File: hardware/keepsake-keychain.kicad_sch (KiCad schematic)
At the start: 3 parts

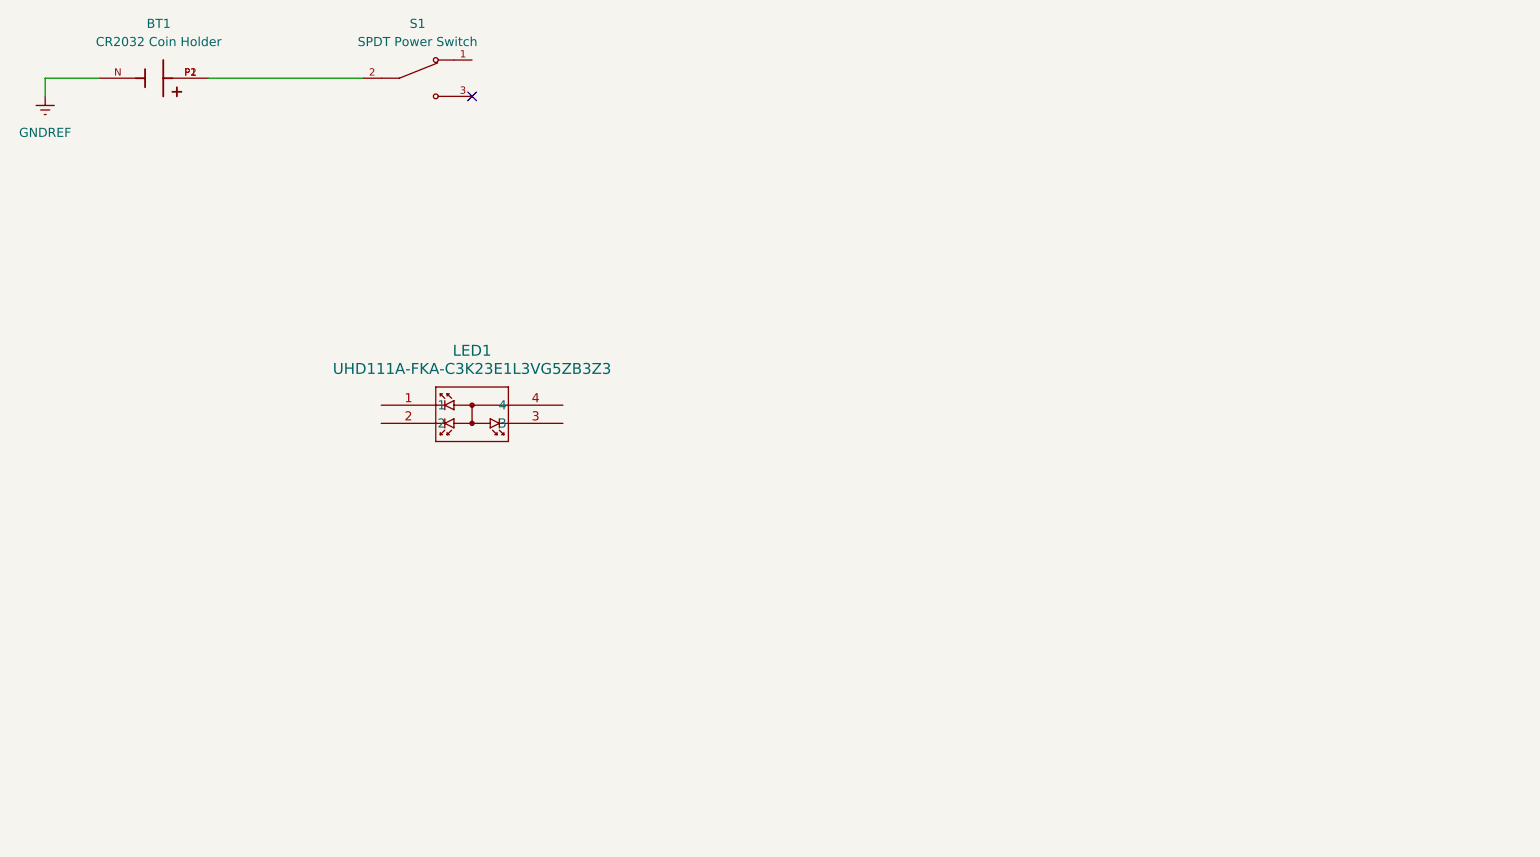
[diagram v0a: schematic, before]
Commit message: Add ATtiny1614 IC
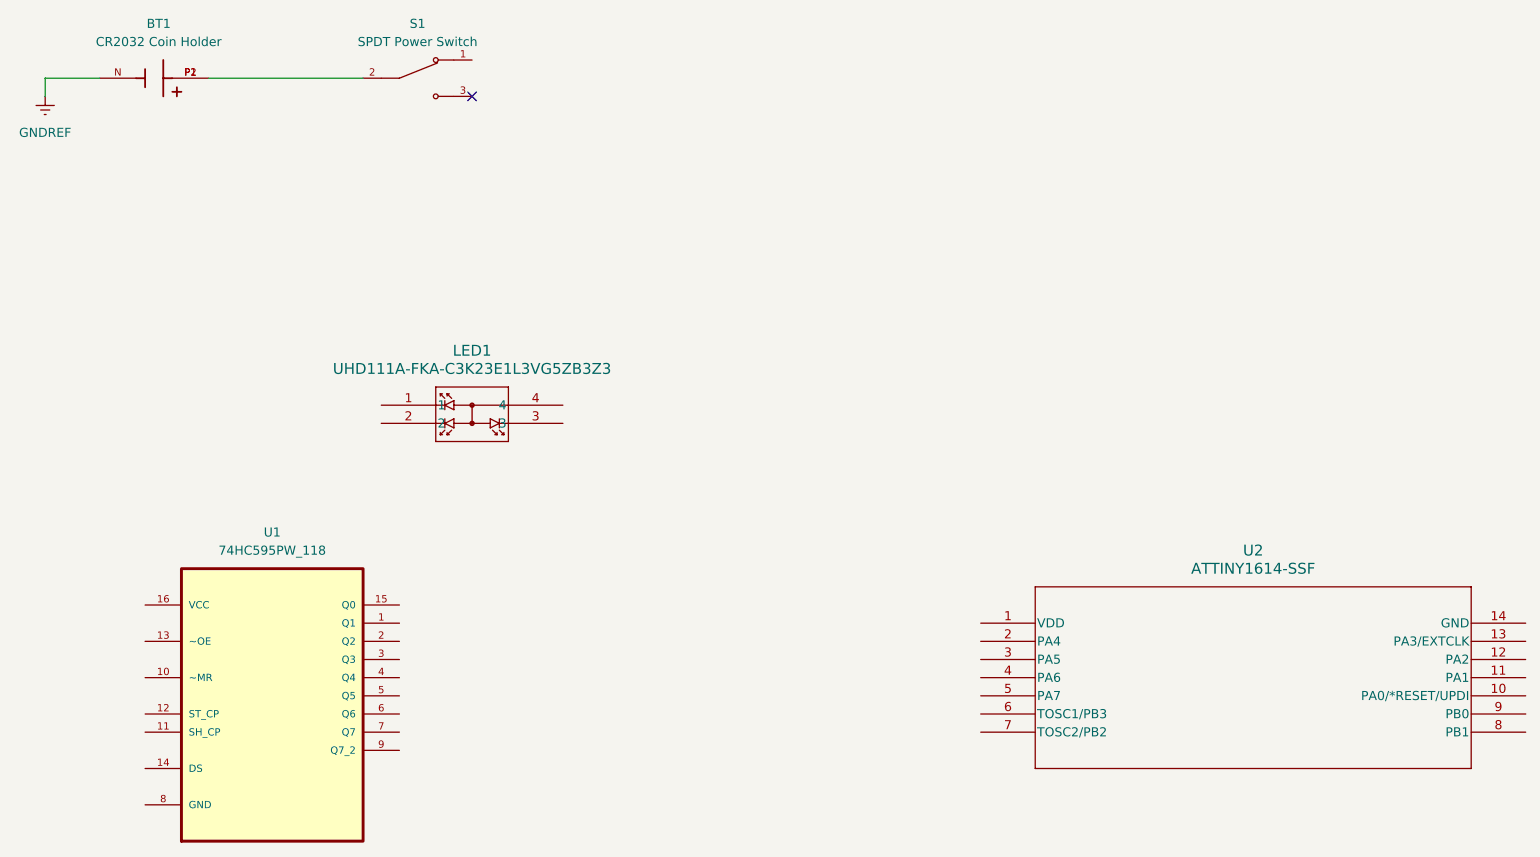
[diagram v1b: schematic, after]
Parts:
- added U1: 74HC595PW_118, 74HC595PW_118:SOP65P640X110-16N, symbol 0_74HC595_Shift_Register:74HC595PW_118
- added U2: ATTINY1614-SSF, SOIC14_SL_MCH, symbol 0_ATtiny1614:ATTINY1614-SSF
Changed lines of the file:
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@@
+	)
+	(symbol
+		(lib_id "0_ATtiny1614:ATTINY1614-SSF")
+		(at 176.53 127 0)
+		(unit 1)
+		(exclude_from_sim no)
+		(in_bom yes)
+		(on_board yes)
+		(dnp no)
+		(fields_autoplaced yes)
+		(property "Reference" "U2"
+			(at 214.63 116.84 0)
+			(effects
+				(font
+					(size 1.524 1.524)
+				)
+			)
+		)
+		(property "Value" "ATTINY1614-SSF"
+			(at 214.63 119.38 0)
+			(effects
+				(font
+					(size 1.524 1.524)
+				)
+			)
+		)
+		(property "Footprint" "SOIC14_SL_MCH"
+			(at 176.53 127 0)
+			(effects
+				(font
+					(size 1.27 1.27)
+					(italic yes)
+				)
+				(hide yes)
+			)
+		)
+		(property "Datasheet" "ATTINY1614-SSF"
+			(at 176.53 127 0)
+			(effects
+				(font
+					(size 1.27 1.27)
+					(italic yes)
+				)
+				(hide yes)
+			)
+		)
+		(property "Description" ""
+			(at 176.53 127 0)
+			(effects
+				(font
+					(size 1.27 1.27)
+				)
+				(hide yes)
+			)
+		)
+		(pin "3"
+		)
+		(pin "1"
+		)
+		(pin "2"
+		)
+		(pin "6"
+		)
+		(pin "8"
+		)
+		(pin "4"
+		)
+		(pin "14"
+		)
+		(pin "12"
+		)
+		(pin "9"
+		)
+		(pin "13"
+		)
+		(pin "10"
+		)
+		(pin "7"
+		)
+		(pin "5"
+		)
+		(pin "11"
+		)
+		(instances
+			(project ""
+				(path "/32670795-e352-430d-9b7f-c7f10ebe6399"
+					(reference "U2")
+					(unit 1)
+				)
+			)
+		)
 	)
 	(symbol
@@
 					(unit 1)
 				)
+			)
+		)
+	)
+	(symbol
+		(lib_id "0_74HC595_Shift_Register:74HC595PW_118")
+		(at 77.47 134.62 0)
+		(unit 1)
+		(exclude_from_sim no)
+		(in_bom yes)
+		(on_board yes)
+		(dnp no)
+		(fields_autoplaced yes)
+		(property "Reference" "U1"
+			(at 77.47 114.3 0)
+			(effects
+				(font
+					(size 1.27 1.27)
+				)
+			)
+		)
+		(property "Value" "74HC595PW_118"
+			(at 77.47 116.84 0)
+			(effects
+				(font
+					(size 1.27 1.27)
+				)
+			)
+		)
+		(property "Footprint" "74HC595PW_118:SOP65P640X110-16N"
+			(at 77.47 134.62 0)
+			(effects
+				(font
+					(size 1.27 1.27)
+				)
+				(justify bottom)
+				(hide yes)
+			)
+		)
+		(property "Datasheet" ""
+			(at 77.47 134.62 0)
+			(effects
+				(font
+					(size 1.27 1.27)
+				)
+				(hide yes)
+			)
+		)
+		(property "Description" ""
+			(at 77.47 134.62 0)
+			(effects
+				(font
+					(size 1.27 1.27)
+				)
+				(hide yes)
+			)
+		)
+		(property "MPN" "74HC595PW,118"
+			(at 77.47 134.62 0)
+			(effects
+				(font
+					(size 1.27 1.27)
+				)
+				(justify bottom)
+				(hide yes)
+			)
+		)
+		(property "OC_FARNELL" "1826846"
+			(at 77.47 134.62 0)
+			(effects
+				(font
+					(size 1.27 1.27)
+				)
+				(justify bottom)
+				(hide yes)
+			)
+		)
+		(property "OC_NEWARK" "78R6263"
+			(at 77.47 134.62 0)
+			(effects
+				(font
+					(size 1.27 1.27)
+				)
+				(justify bottom)
+				(hide yes)
+			)
+		)
+		(property "SUPPLIER" "NXP"
+			(at 77.47 134.62 0)
+			(effects
+				(font
+					(size 1.27 1.27)
+				)
+				(justify bottom)
+				(hide yes)
+			)
+		)
+		(property "PACKAGE" "TSSOP-16"
+			(at 77.47 134.62 0)
+			(effects
+				(font
+					(size 1.27 1.27)
+				)
+				(justify bottom)
+				(hide yes)
+			)
+		)
+		(pin "3"
+		)
+		(pin "8"
+		)
+		(pin "12"
+		)
+		(pin "13"
+		)
+		(pin "16"
+		)
+		(pin "10"
+		)
+		(pin "11"
+		)
+		(pin "14"
+		)
+		(pin "1"
+		)
+		(pin "15"
+		)
+		(pin "2"
+		)
+		(pin "4"
+		)
+		(pin "5"
+		)
+		(pin "6"
+		)
+		(pin "9"
+		)
+		(pin "7"
+		)
+		(instances
+			(project ""
+				(path "/32670795-e352-430d-9b7f-c7f10ebe6399"
+					(reference "U1")
+					(unit 1)
+				)
